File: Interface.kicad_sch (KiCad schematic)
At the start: 44 parts, among them J6301 PV, J6302 PV, J6303 VBUS, J6304 PV, J6305 PV, J6306 PV, J6307 PV, J6308 Chan, J6309 Chan, J6310 Chan, J6311 Chan, J6312 Chan, J6313 Chan, J6314 Chan, J6315 Chan, J6316 Chan_BUS, J6317 Chan_BUS, J6318 VBUS, J6319 VBUS, J6320 Battery, J6321 Battery, J6322 HEADER_PV, J6323 HEADER_PV, J6324 HEADER_CHAN, J6325 HEADER_CHAN, J6326 HEADER_CHAN, J6327 HEADER_CHAN, J6328 VBUS, J6329 SPI, J6330 UART

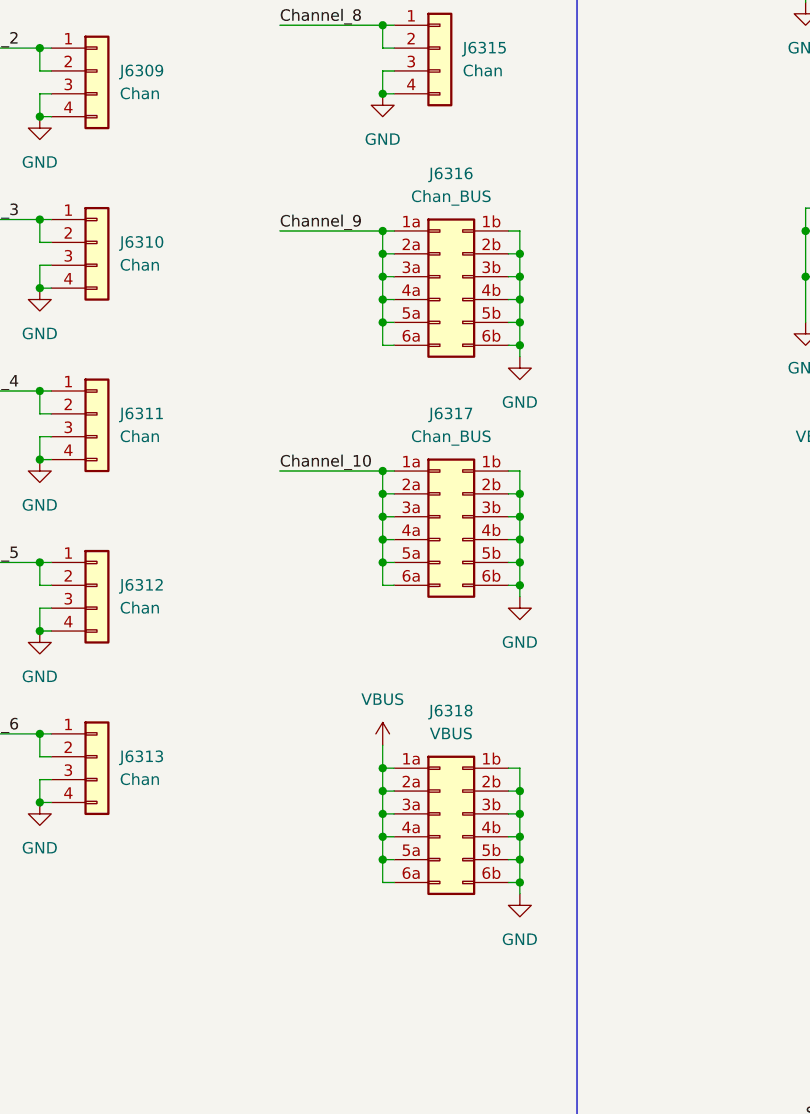
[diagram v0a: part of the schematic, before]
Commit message: minor adjustments
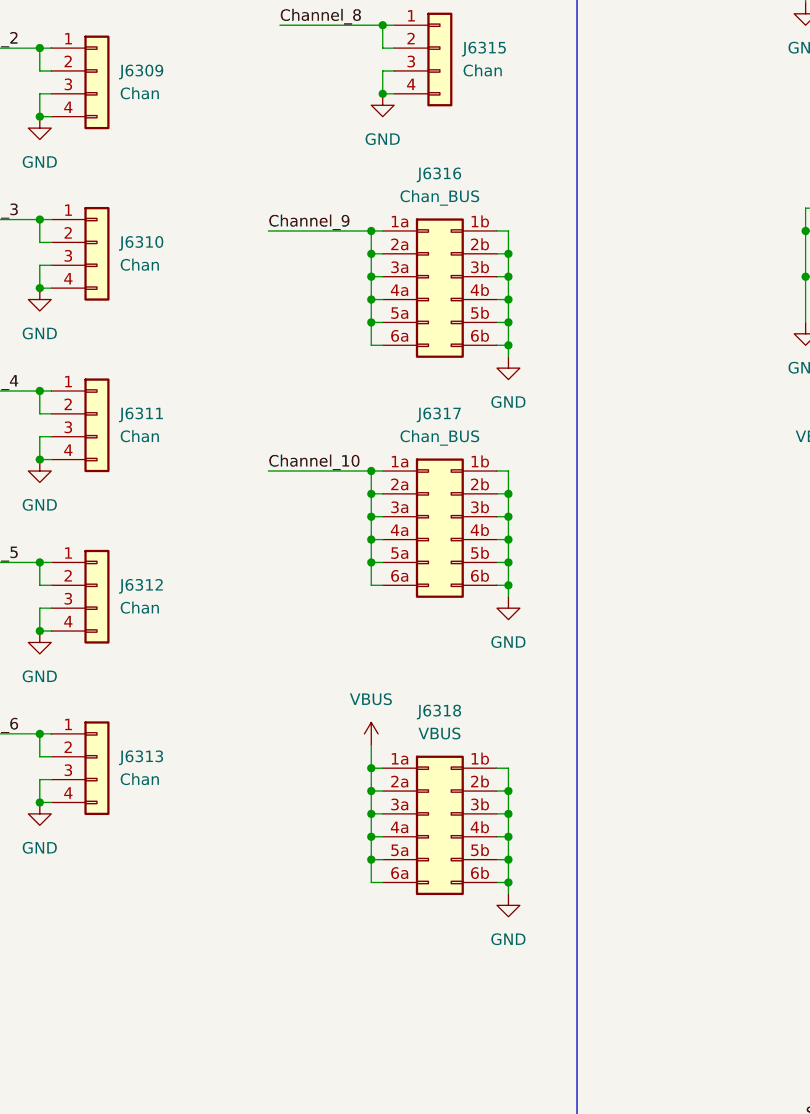
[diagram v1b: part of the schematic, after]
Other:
- moved on the sheet: J6316, J6317, J6318
